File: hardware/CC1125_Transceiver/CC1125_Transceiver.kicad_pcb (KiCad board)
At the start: 4 copper layers, 53.7 x 25.1 mm, 75 parts, among them IC1 CC1125RHBT, IC2 GALI-74+, IC3 TLV61046ADBVT, IC4 TLV75801PDRVR, J1 SMA_Ant, J2 Conn_02x03_Counter_Clockwise, J4 USB_C_Receptacle_USB2.0_14P, U2 STM32L412K8Ux, Y1 ECS-TXO-32CSMV-400-BN-TR, Y2 40MHz

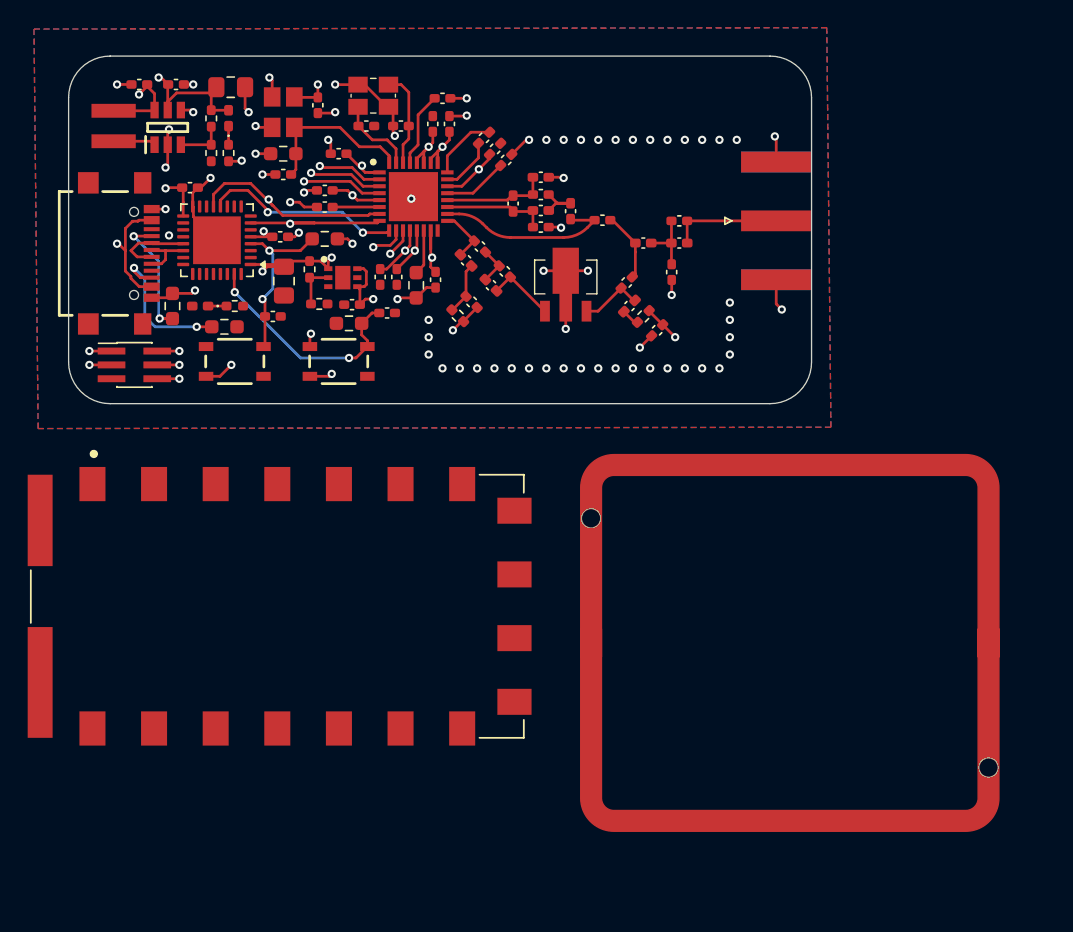
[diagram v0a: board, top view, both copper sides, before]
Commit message: updated
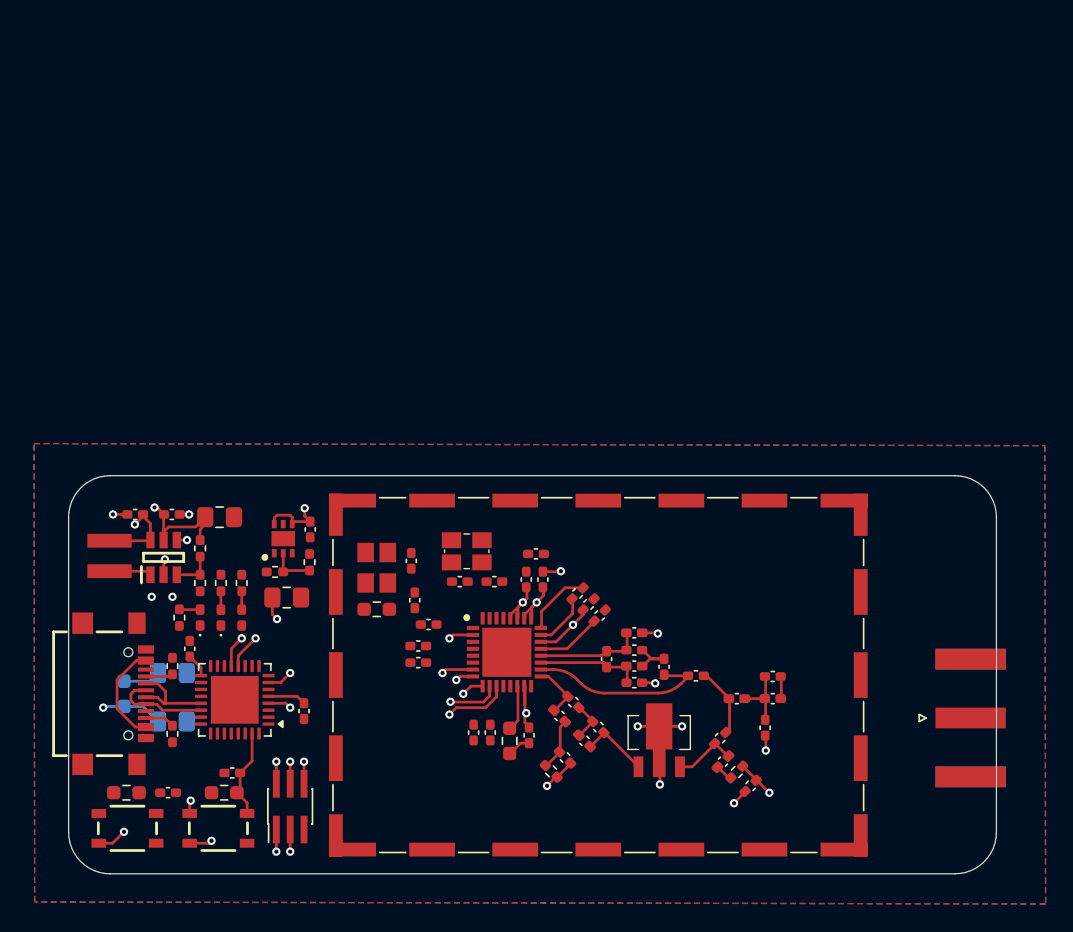
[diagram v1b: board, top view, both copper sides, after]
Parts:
- removed REF**: ${Value}, libary:VHF_UHF_Module_generic
- added C36: DNP, Capacitor_SMD:C_0805_2012Metric_Pad1.18x1.45mm_HandSolder, B.Cu at (84.0, 96.0)
- added C37: DNP, Capacitor_SMD:C_0805_2012Metric_Pad1.18x1.45mm_HandSolder, B.Cu at (84.0, 99.5)
- added D4: ~, LED_SMD:LED_0402_1005Metric_Pad0.77x0.64mm_HandSolder, F.Cu at (89.0, 92.0)
- added R15: 5.1k, Resistor_SMD:R_0402_1005Metric_Pad0.72x0.64mm_HandSolder, F.Cu at (89.0, 89.5)
- added R16: 0, Resistor_SMD:R_0603_1608Metric_Pad0.98x0.95mm_HandSolder, B.Cu at (80.5, 97.5)
- H2: value 3670288 -> 3610637256S; footprint libary:H_Wurth_WE-SHC-SEAMLESS-FRAME_3670290 -> SHIELDING_SMD_Wurth:H_Wurth_WE-SHC-SMT-FRAME_3610637256S
- R6, R7: footprint Resistor_SMD:R_0603_1608Metric_Pad0.98x0.95mm_HandSolder -> Resistor_SMD:R_0402_1005Metric_Pad0.72x0.64mm_HandSolder
- moved R10 42.5 mm to (80.7, 104.6), turned to 0 degrees
- moved J1 38.5 mm to (141.6, 99.2)
- moved D3 36.1 mm to (87.5, 92.0)
- moved C31 35.2 mm to (83.7, 104.6)
- moved R13 35.1 mm to (87.7, 104.6)
- moved C33 35.0 mm to (88.3, 103.2), turned to 180 degrees
- moved Boot1 34.8 mm to (87.3, 107.2)
- moved C20 34.6 mm to (102.5, 92.5)
- moved Reset1 34.6 mm to (80.8, 107.2)
- moved C1 34.3 mm to (93.5, 98.8), turned to -90 degrees
- moved J2 33.8 mm to (92.5, 105.7), turned to 90 degrees
- moved C10 33.6 mm to (125.8, 104.2)
- moved C11 33.6 mm to (123.5, 100.7)
- moved C13 33.6 mm to (109.8, 100.5)
- moved C24 33.6 mm to (110.2, 87.4)
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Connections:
- D2 pad 1: Net-(D2-K) -> GND
- D2 pad 2: unconnected-(D2-A-Pad2) -> Net-(D2-A)
- D3 pad 1: Net-(D3-K) -> GND
- D3 pad 2: +7V -> Net-(D3-A)
- J4 pad A4: VUSB -> Net-(C37-Pad1)
- J4 pad B4: VUSB -> Net-(C37-Pad1)
- R11 pad 1: Net-(D2-K) -> unconnected-(R11-Pad1)
- R11 pad 2: GND -> Net-(D2-A)
- R12 pad 1: Net-(D3-K) -> +7V
- R12 pad 2: GND -> Net-(D3-A)
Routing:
- net +7V: track 71.0 -> 12.0 mm
- net +3V3: track 83.3 -> 26.8 mm, vias 16 -> 7
- net VUSB: track 60.1 -> 14.2 mm, vias 5 -> 3
- net GND: track 59.8 -> 18.7 mm, vias 72 -> 15
- net /SPI_MOSI: track 34.3 -> 6.21 mm, vias 2 -> 3
- net /SPI_MISO: track 33.2 -> 5.75 mm
- net /SPI_SCK: track 31.5 -> 4.75 mm, vias 2 -> 3
- net /CC_Resetn: track 24.5 -> 3.40 mm
- net /SPI_CSN: track 22.6 -> 6.30 mm
- net Net-(C37-Pad1): track 0.00 -> 12.3 mm, vias 0 -> 1
- net Net-(IC1-EXT_XOSC): track 11.8 -> 0.00 mm
- net /uc_Reset: track 12.7 -> 2.05 mm, vias 2 -> 1
- net /uc_Boot: track 16.9 -> 6.76 mm, vias 2 -> 0
- net Net-(J4-CC2): track 10.7 -> 2.14 mm, vias 2 -> 0
- net Net-(J4-CC1): track 9.12 -> 1.98 mm, vias 2 -> 0
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- removed copper zone on In2.Cu, net +3V3
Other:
- board size 53.7 x 25.1 mm -> 67 x 28.8 mm
- board text added: "<GHz Trans ceiver"
- board text added: "PA"
- board text added: "V1.0 Gewiese"
- board text added: "VCC"
- board text added: "rst"
- board text added: "uC"
- board text removed: "50Ω"
- board text removed: "Sub GHz RF Transceiver"
- board text removed: "V1.0 Fynn Gewiese"
- board text removed: "reset"
